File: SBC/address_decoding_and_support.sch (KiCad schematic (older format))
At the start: 15 parts, among them Q1 DS1813, SW1 RESET, SW2 PANIC, U5 TL7705B, U6 PlutoDecoder, U8 74HC74, X1 8MHz

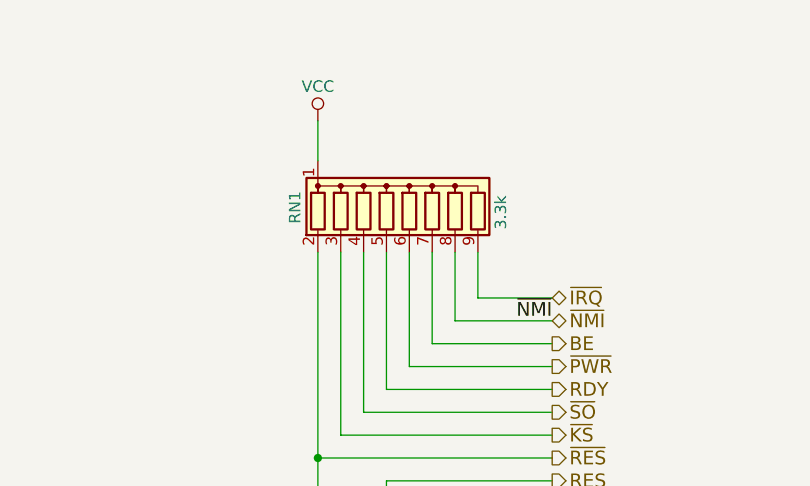
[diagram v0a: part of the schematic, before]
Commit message: New PCB layout is taking shape.
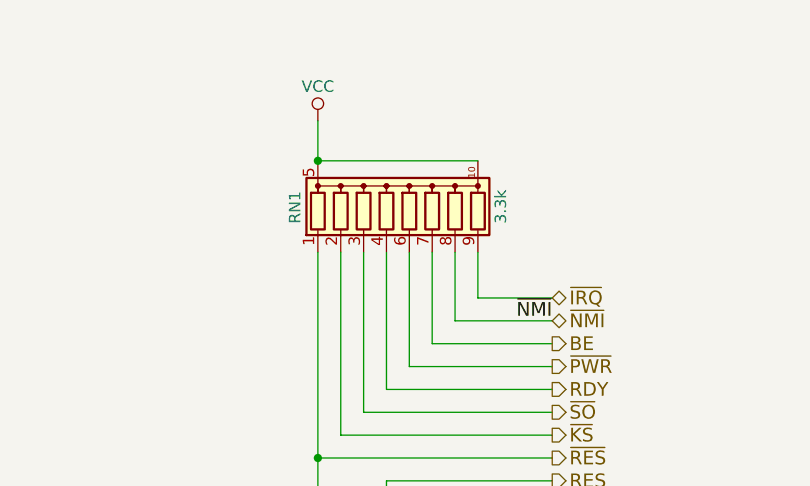
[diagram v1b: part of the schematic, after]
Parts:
- removed RN1: 3.3k, Resistor_SMD:R_Array_Convex_8x0602, symbol Device:R_Network08
- added RN1: 3.3k, Resistor_SMD:R_Array_Convex_5x1206, symbol Grotto:R_Network08_SMD
- C10, C6, C9: footprint Capacitor_SMD:C_0603_1608Metric_Pad1.05x0.95mm_HandSolder -> Capacitor_SMD:C_0805_2012Metric_Pad1.15x1.40mm_HandSolder
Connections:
- net BE: now also RN1.7 (R6)
- net RDY: now also RN1.4 (R4)
- net VCC: now also RN1.10 (common), RN1.5 (common)
- net ~IRQ: now also RN1.9 (R8)
- net ~KS: now also RN1.2 (R2)
- net ~NMI: now also RN1.8 (R7)
- net ~PWR: now also RN1.6 (R5)
- net ~RES: now also RN1.1 (R1)
- net ~SO: now also RN1.3 (R3)
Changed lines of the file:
@@
 F 0 "C6" H 3650 3700 50  0000 L CNN
 F 1 "0.1uF" H 3425 3550 50  0000 L CNN
-F 2 "Capacitor_SMD:C_0603_1608Metric_Pad1.05x0.95mm_HandSolder" H 3650 3625 50  0001 C CNN
+F 2 "Capacitor_SMD:C_0805_2012Metric_Pad1.15x1.40mm_HandSolder" H 3650 3625 50  0001 C CNN
 F 3 "" H 3650 3625 50  0001 C CNN
 	1    3650 3625
@@
 	4350 1800 4675 1800
 Wire Wire Line
-	3650 1200 3650 1025
-Wire Wire Line
 	4650 6450 4900 6450
 Wire Wire Line
@@
 Wire Wire Line
 	3750 2400 4675 2400
-$Comp
-L Device:R_Network08 RN1
-U 1 1 5D76ADD1
-P 4050 1400
-F 0 "RN1" V 3550 1325 50  0000 L CNN
-F 1 "3.3k" V 4450 1300 50  0000 L CNN
-F 2 "Resistor_SMD:R_Array_Convex_8x0602" V 4525 1400 50  0001 C CNN
-F 3 "http://www.vishay.com/docs/31509/csc.pdf" H 4050 1400 50  0001 C CNN
-	1    4050 1400
-	1    0    0    -1
-$EndComp
 Wire Wire Line
 	4675 2500 3650 2500
@@
 F 0 "C9" V 8775 800 50  0000 C CNN
 F 1 "0.1uF" V 9025 800 50  0000 C CNN
-F 2 "Capacitor_SMD:C_0603_1608Metric_Pad1.05x0.95mm_HandSolder" H 8900 800 50  0001 C CNN
+F 2 "Capacitor_SMD:C_0805_2012Metric_Pad1.15x1.40mm_HandSolder" H 8900 800 50  0001 C CNN
 F 3 "~" H 8900 800 50  0001 C CNN
 	1    8900 800
@@
 F 0 "C10" V 3775 6775 50  0000 L CNN
 F 1 "0.1uF" V 4000 6750 50  0000 L CNN
-F 2 "Capacitor_SMD:C_0603_1608Metric_Pad1.05x0.95mm_HandSolder" H 3875 6825 50  0001 C CNN
+F 2 "Capacitor_SMD:C_0805_2012Metric_Pad1.15x1.40mm_HandSolder" H 3875 6825 50  0001 C CNN
 F 3 "" H 3875 6825 50  0001 C CNN
 	1    3875 6825
@@
 	3775 6150 4050 6150
 Connection ~ 4050 6150
+$Comp
+L Grotto:R_Network08_SMD RN1
+U 1 1 5D847681
+P 4050 1400
+F 0 "RN1" V 3550 1325 50  0000 L CNN
+F 1 "3.3k" V 4450 1325 50  0000 L CNN
+F 2 "Resistor_SMD:R_Array_Convex_5x1206" V 4525 1400 50  0001 C CNN
+F 3 "https://industrial.panasonic.com/cdbs/www-data/pdf/AOC0000/AOC0000C12.pdf" H 4050 1400 50  0001 C CNN
+	1    4050 1400
+	1    0    0    -1
+$EndComp
+Wire Wire Line
+	3650 1200 3650 1025
+Wire Wire Line
+	4350 1200 3650 1200
+Connection ~ 3650 1200
 Wire Bus Line
 	7375 1025 7375 2025
